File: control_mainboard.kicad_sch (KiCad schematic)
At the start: 61 parts, among them J201 USB_C_Receptacle_USB2.0_14P, J202 SD_Card_Receptacle, J203 [battery], J204 FFC Connector, J205 SM03B-SRSS-TB, Q201 DMG3415, Q202 DMG3415, SW201 [bootstrap button], SW202 [reset button], SW203 SW_SPST, U201 MCP73831-2-OT, U202 XC6220B331MR, U203 W25Q128JVS, U204 RP2350A, U205 74AHC1G04, U206 W25Q128JVS, Y201 ABM8-272-T3

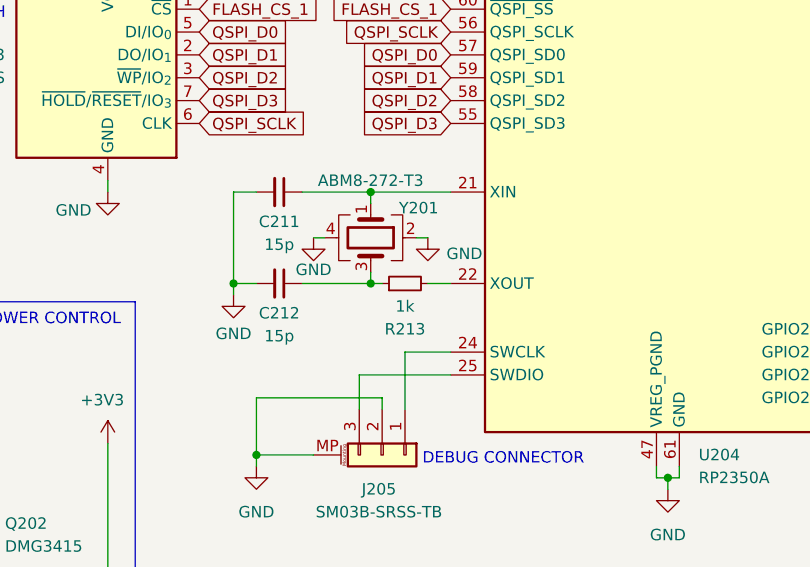
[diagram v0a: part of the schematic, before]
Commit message: crystal oscillator
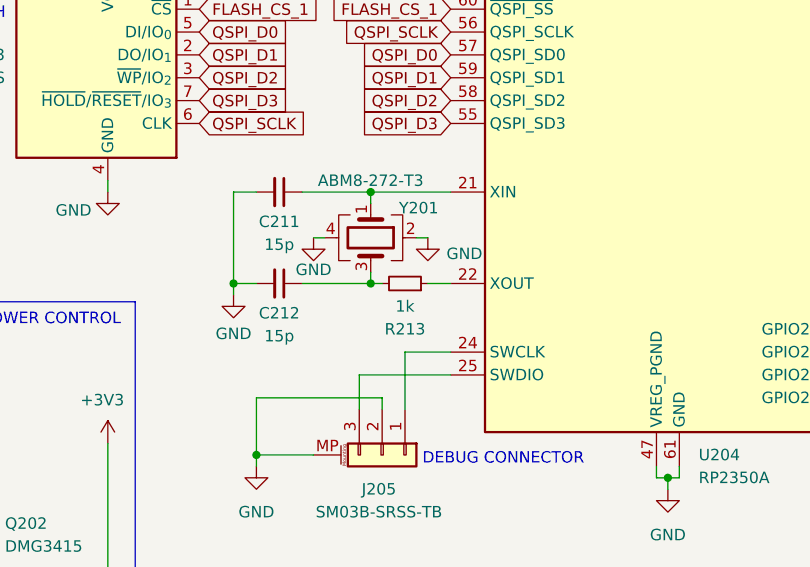
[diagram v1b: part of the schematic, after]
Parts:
- C211, C212: footprint Capacitor_SMD:C_0805_2012Metric -> Capacitor_SMD:C_0402_1005Metric
- R213: footprint Resistor_SMD:R_1206_3216Metric -> Resistor_SMD:R_0402_1005Metric
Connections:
- net at C212.1, Y201.3: now also R213.2; no longer R213.1
- net at U204.22 (XOUT): now also R213.1; no longer R213.2
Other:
- moved on the sheet: R213
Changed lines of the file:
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@@
 			)
 		)
-		(property "Footprint" "Capacitor_SMD:C_0805_2012Metric"
+		(property "Footprint" "Capacitor_SMD:C_0402_1005Metric"
 			(at 148.59 119.38 0)
 			(hide yes)
@@
 			)
 		)
-		(property "Footprint" "Capacitor_SMD:C_0805_2012Metric"
+		(property "Footprint" "Capacitor_SMD:C_0402_1005Metric"
 			(at 148.59 129.54 0)
 			(hide yes)
@@
 	(symbol
 		(lib_id "Device:R_Small")
-		(at 162.56 129.54 90)
+		(at 162.56 129.54 270)
+		(mirror x)
 		(unit 1)
 		(body_style 1)
@@
 			)
 		)
-		(property "Footprint" "Resistor_SMD:R_1206_3216Metric"
+		(property "Footprint" "Resistor_SMD:R_0402_1005Metric"
 			(at 162.56 129.54 0)
 			(hide yes)
